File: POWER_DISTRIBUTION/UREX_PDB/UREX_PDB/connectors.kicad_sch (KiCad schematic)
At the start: 23 parts, among them J10 Conn_01x02, J11 Conn_01x02, J28 Conn_01x06, J30 Conn_01x02, J31 Conn_01x02, J32 Conn_01x04, J33 Conn_01x02, J34 Conn_01x02, J35 Conn_01x03, J36 Conn_01x03, J8 Conn_01x02, J9 Conn_01x02, U7 USBLC6-2SC6

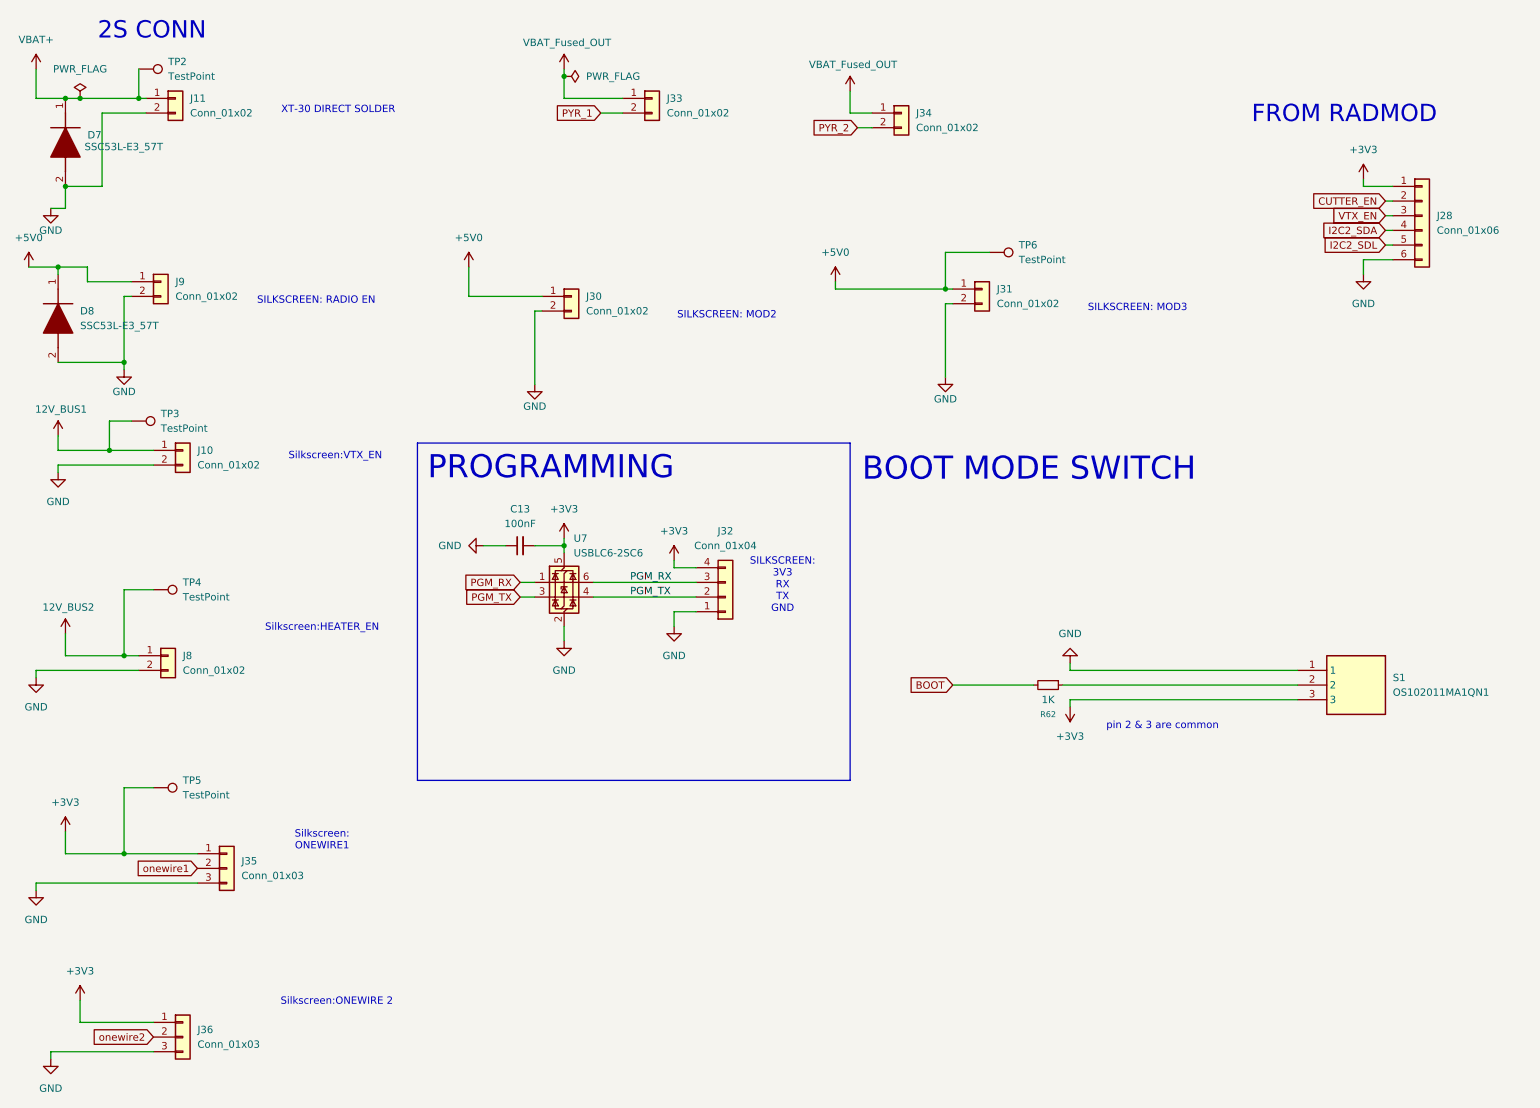
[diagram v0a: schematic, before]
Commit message: FIXED LIBRARY
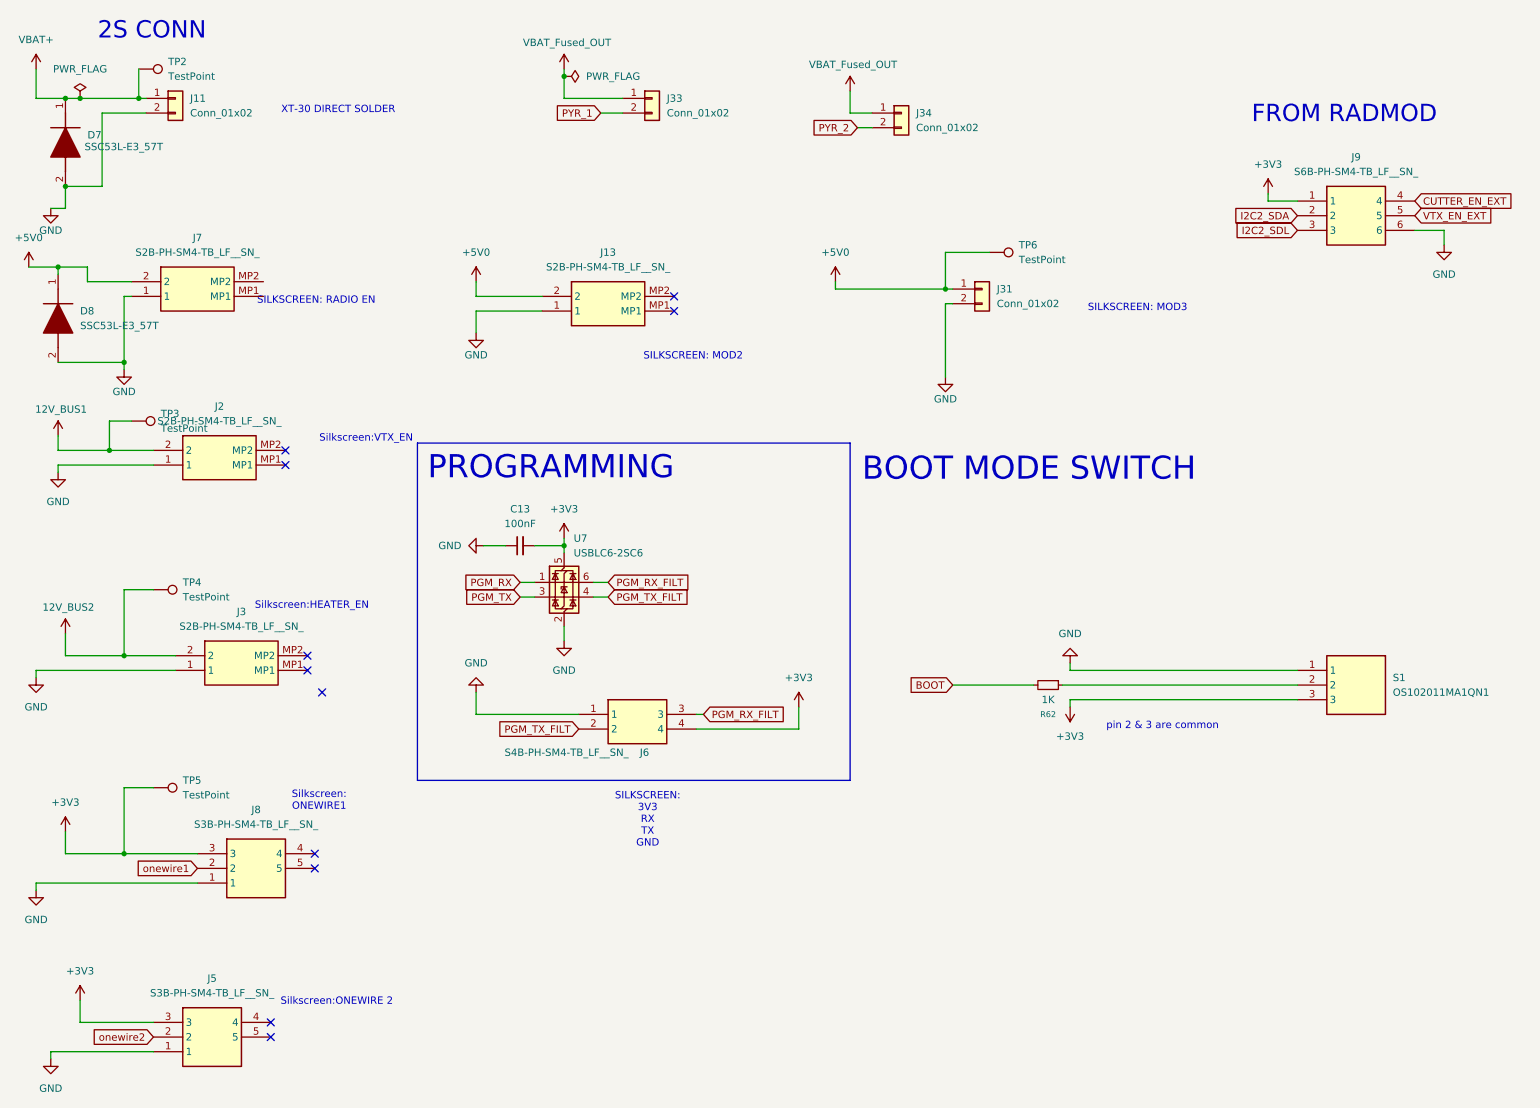
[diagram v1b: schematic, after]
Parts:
- removed J10, J8, J9: Conn_01x02, Connector_JST:JST_PH_S2B-PH-K_1x02_P2.00mm_Horizontal, symbol Connector_Generic:Conn_01x02
- removed J28: Conn_01x06, Connector_JST:JST_PH_S6B-PH-K_1x06_P2.00mm_Horizontal, symbol Connector_Generic:Conn_01x06
- removed J30: Conn_01x02, Connector_JST:JST_PH_B2B-PH-K_1x02_P2.00mm_Vertical, symbol Connector_Generic:Conn_01x02
- removed J32: Conn_01x04, Connector_JST:JST_PH_S4B-PH-K_1x04_P2.00mm_Horizontal, symbol Connector_Generic:Conn_01x04
- removed J35, J36: Conn_01x03, Connector_JST:JST_PH_S3B-PH-K_1x03_P2.00mm_Horizontal, symbol Connector_Generic:Conn_01x03
- added J13, J2, J3, J7: S2B-PH-SM4-TB_LF__SN_, SamacSys_Parts:S2BPHSM4TBLFSN, symbol SamacSys_Parts:S2B-PH-SM4-TB_LF__SN_
- added J5, J8: S3B-PH-SM4-TB_LF__SN_, SamacSys_Parts:S3BPHSM4TBLFSN, symbol SamacSys_Parts:S3B-PH-SM4-TB_LF__SN_
- added J6: S4B-PH-SM4-TB_LF__SN_, SamacSys_Parts:S4B-PH-SM4-TB, symbol SamacSys_Parts:S4B-PH-SM4-TB_LF__SN_
- added J9: S6B-PH-SM4-TB_LF__SN_, S6B-PH-SM4-TB(LF)(SN)_3, symbol SamacSys_Parts:S6B-PH-SM4-TB_LF__SN_
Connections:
- net +3V3: now also J5.3, J6.4, J8.3, J9.1
- net +5V0: now also J13.2, J7.2
- net 12V_BUS1: now also J2.2
- net 12V_BUS2: now also J3.2
- net GND: now also J13.1, J2.1, J3.1, J5.1, J6.1, J7.1, J8.1, J9.6
- net I2C2_SDA: now also J9.2
- net I2C2_SDL: now also J9.3
- net PGM_RX: no longer U7.6 (I/O1)
- net PGM_TX: no longer U7.4 (I/O2)
- net onewire1: now also J8.2
- net onewire2: now also J5.2
- new net CUTTER_EN_EXT: J9.4
- new net PGM_RX_FILT: J6.3, U7.6 (I/O1)
- new net PGM_TX_FILT: J6.2, U7.4 (I/O2)
- new net VTX_EN_EXT: J9.5
- no-connect marks 0 -> 11
